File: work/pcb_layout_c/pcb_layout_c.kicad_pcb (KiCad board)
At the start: 2 copper layers, 15 parts, among them J1 Conn_01x15_Pin

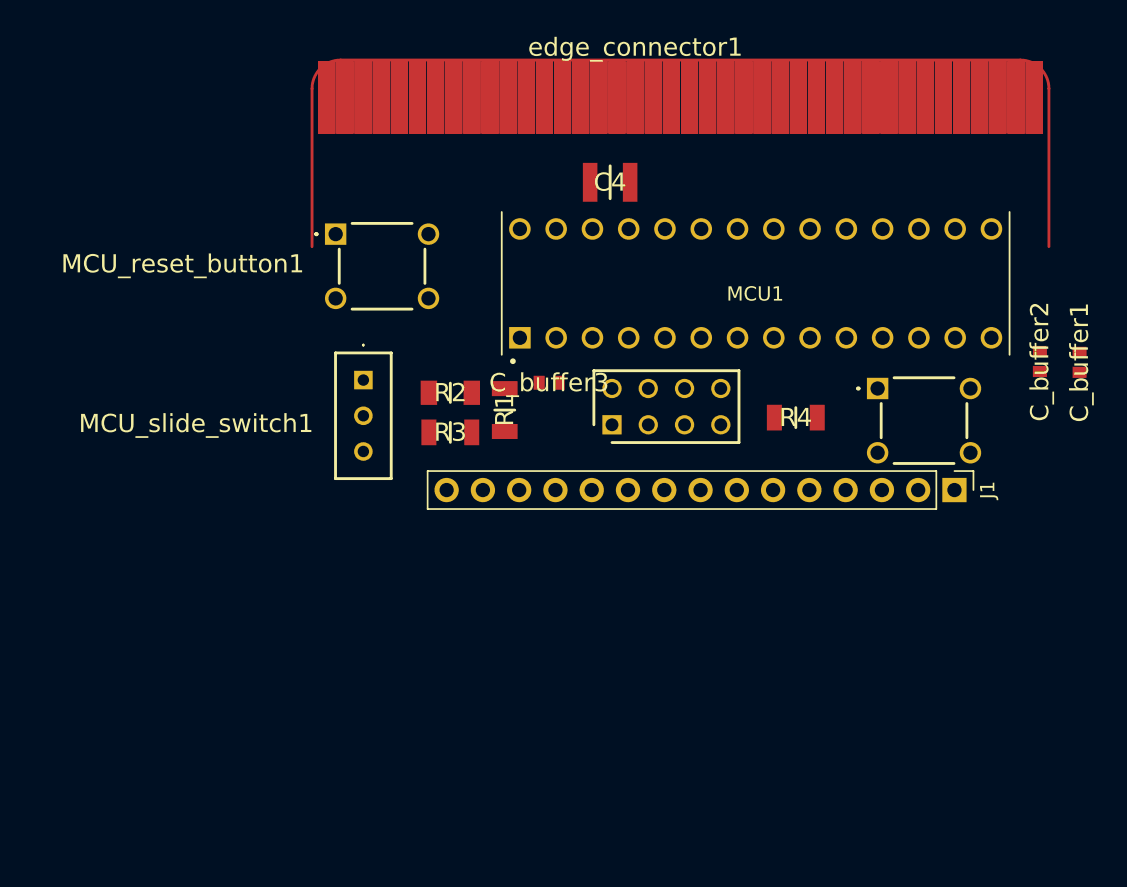
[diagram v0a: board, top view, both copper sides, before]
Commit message: Issue #22 : Kreiranje PCB dizajna cjelokupnog sistema
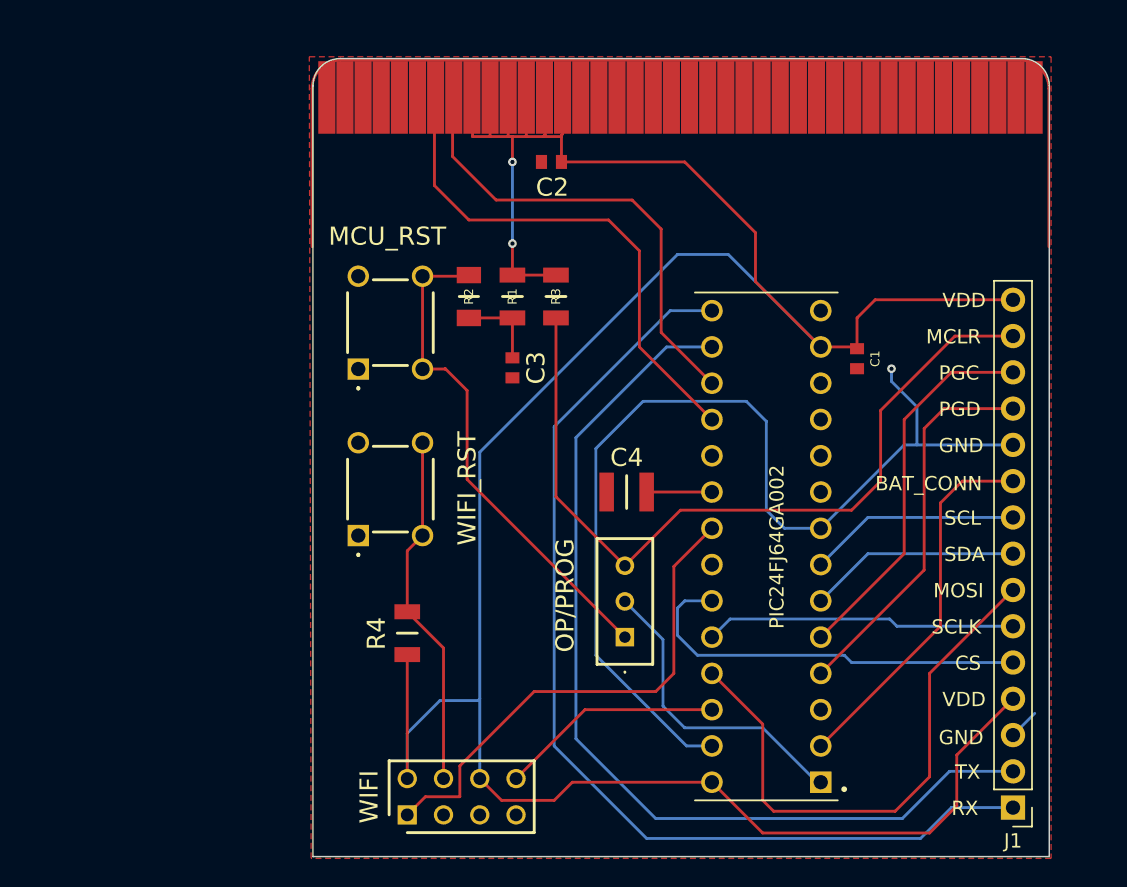
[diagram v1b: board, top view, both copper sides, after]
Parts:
- moved WIFI_RST 37.8 mm to (90.0, 128.8), turned to 90 degrees
- moved C2 36.9 mm to (103.6, 102.6), turned to 180 degrees
- moved R4 31.1 mm to (93.5, 135.6), turned to 90 degrees
- moved WIFI 30.9 mm to (93.5, 148.3)
- moved OP/PROG 25.7 mm to (108.7, 135.9), turned to 90 degrees
- moved J1 22.6 mm to (135.9, 147.8), turned to 180 degrees
- moved C4 21.7 mm to (108.8, 125.7)
- moved PIC24FJ64GA002 18.4 mm to (118.6, 129.5), turned to 180 degrees
- moved C1 15.6 mm to (125.0, 116.4)
- moved R3 12.0 mm to (103.9, 112.0), turned to 90 degrees
- moved MCU_RST 9.58 mm to (90.0, 117.1), turned to 90 degrees
- moved R1 7.97 mm to (100.8, 112.0), turned to 90 degrees
- moved R2 6.87 mm to (97.8, 112.0), turned to 90 degrees
- moved C3 2.78 mm to (100.8, 117.0), turned to -90 degrees
- renumbered C_buffer1 to C1, C_buffer2 to C2, C_buffer3 to C3, MCU_reset_button1 to MCU_RST, MCU_slide_switch1 to OP/PROG, MCU1 to PIC24FJ64GA002, WiFi_socket1 to WIFI, WiFi_reset_button1 to WIFI_RST
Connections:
- OP/PROG pad 1: unconnected-(MCU_slide_switch1-NC-Pad1) -> Net-(MCU_reset_button1-COM_1)
- WIFI pad 1: GND -> RX input
- WIFI pad 2: TX out -> VDD
- WIFI pad 4: VDD -> Net-(WiFi_reset_button1-COM_1)
- WIFI pad 6: Net-(WiFi_reset_button1-COM_1) -> VDD
- WIFI pad 7: RX input -> GND
- WIFI pad 8: VDD -> TX out
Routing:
- net VDD: track 0.00 -> 198.1 mm, vias 0 -> 2
- net GND: track 0.00 -> 73.8 mm, vias 0 -> 1
- net RX: track 0.00 -> 72.5 mm
- net TX: track 0.00 -> 67.5 mm
- net MCLR: track 0.00 -> 56.1 mm
- net SPI1 Data Output: track 0.00 -> 38.9 mm
- net Net-(MCU1-TDO/RP9/SDA1/CN21/PMD3/RB9): track 0.00 -> 36.4 mm
- net Net-(MCU_reset_button1-COM_1): track 0.00 -> 35.4 mm
- net RX input: track 0.00 -> 35.3 mm
- net Net-(MCU1-TCK/RP8/SCL1/CN22/PMD4/RB8): track 0.00 -> 33.1 mm
- net SPI1 Slave Select Output: track 0.00 -> 28.8 mm
- net PGD1: track 0.00 -> 26.9 mm
- net PGC1: track 0.00 -> 26.6 mm
- net BAT_CONN: track 0.00 -> 26.2 mm
- net Net-(WiFi_reset_button1-COM_1): track 0.00 -> 25.0 mm
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- added copper zone on F.Cu, net GND
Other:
- board outline added: 51.6 x 55.9 mm
- board text added: "Anja Đaković"
- board text added: "BAT_CONN"
- board text added: "CS"
- board text added: "GND"
- board text added: "Grupa C:"
- board text added: "MCLR"
- board text added: "MOSI"
- board text added: "Nikola Babić"
- board text added: "PGC"
- board text added: "PGD"
- board text added: "RX"
- board text added: "Radislav Kosijer"
- board text added: "SCL"
- board text added: "SCLK"
- board text added: "SDA"
- board text added: "TX"
- board text added: "VDD"
